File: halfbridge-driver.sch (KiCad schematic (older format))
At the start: 33 parts, among them U12 MGJ1, U13 MGJ1, U14 2ED020I12-F2

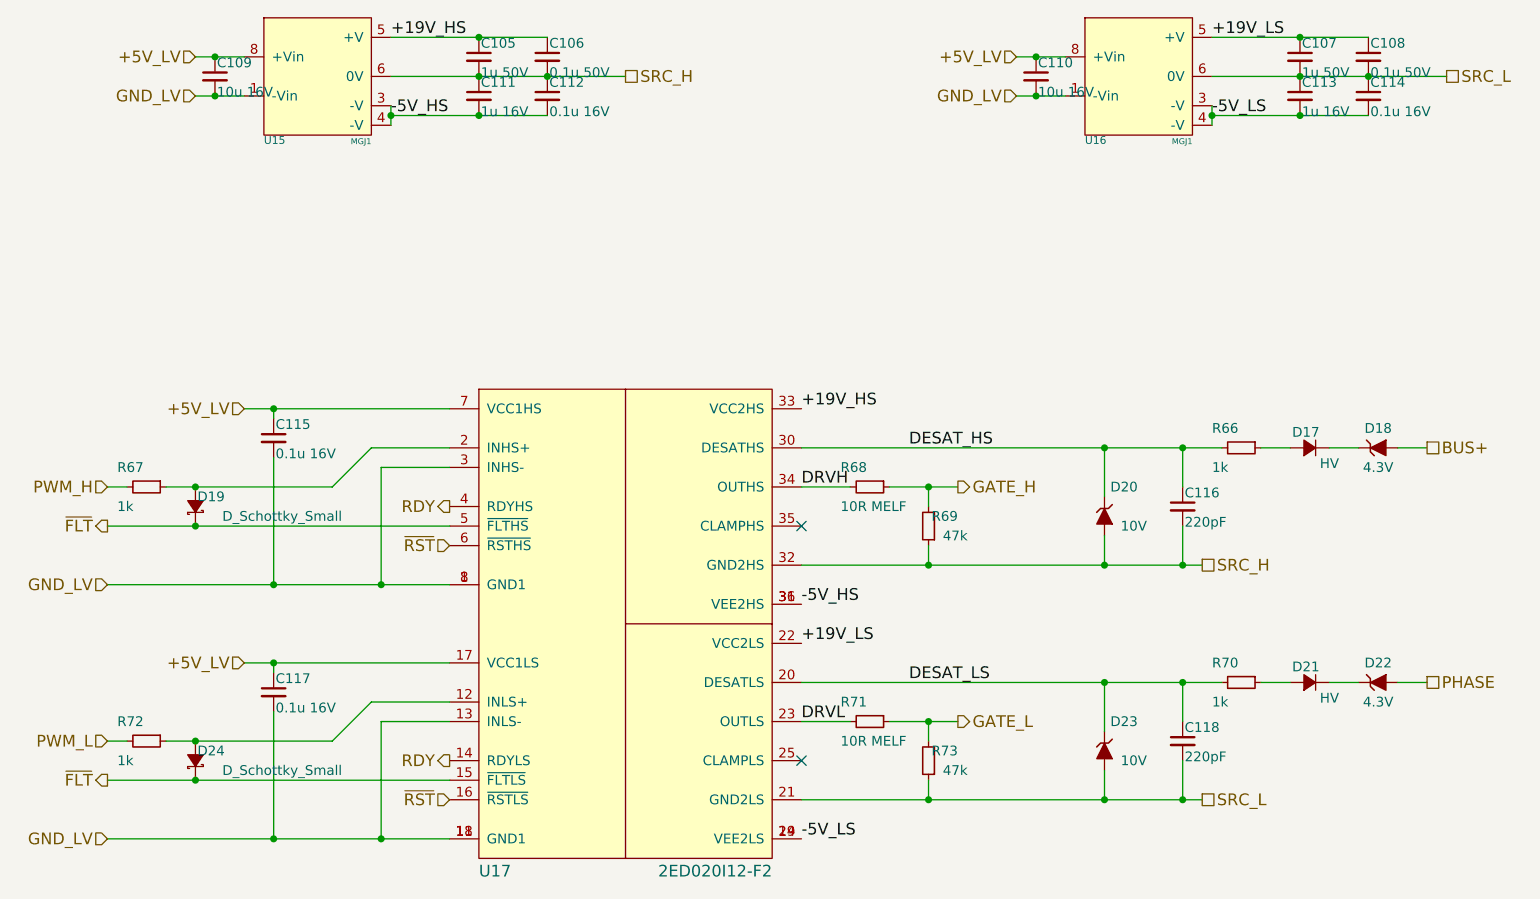
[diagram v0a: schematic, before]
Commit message: Add aux connector for vibe monitor
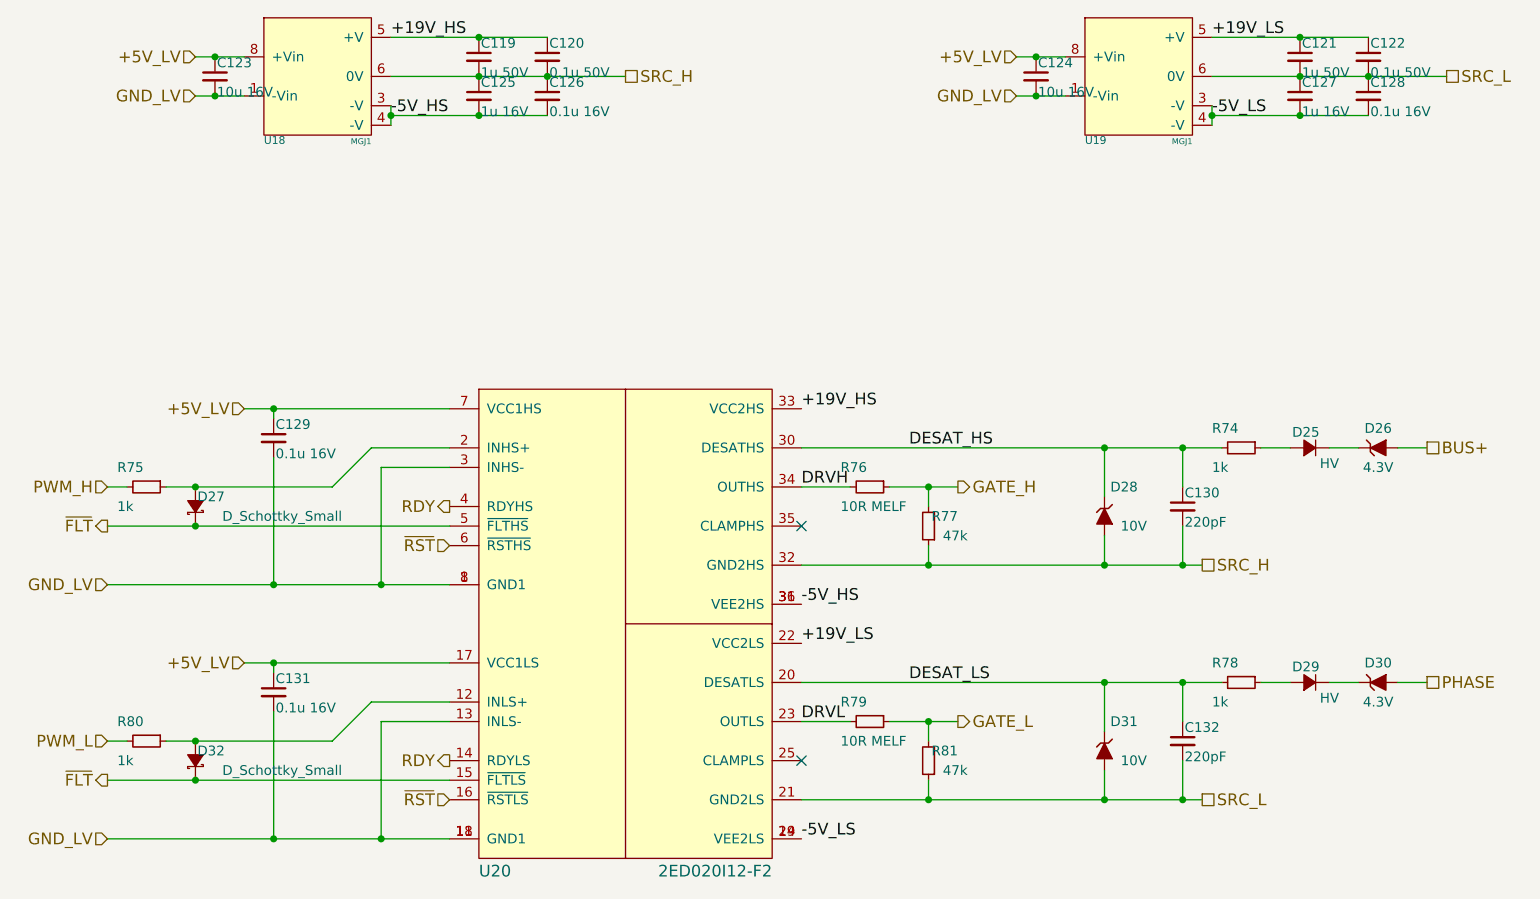
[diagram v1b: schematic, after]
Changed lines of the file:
@@
 AR Path="/57A1662D/57F260F4/57F02200" Ref="U17"  Part="1"
 AR Path="/57A1662D/57F2705F/57F02200" Ref="U20"  Part="1"
-F 0 "U17" H 4450 2750 60  0000 L BNN
+F 0 "U20" H 4450 2750 60  0000 L BNN
 F 1 "2ED020I12-F2" H 5950 2750 60  0000 R BNN
 F 2 "sictroller:PG-DSO-36-58" H 5200 4050 60  0001 C CNN
@@
 AR Path="/57A1662D/57F260F4/57F05C45" Ref="U15"  Part="1"
 AR Path="/57A1662D/57F2705F/57F05C45" Ref="U18"  Part="1"
-F 0 "U15" H 3350 900 40  0000 L BNN
+F 0 "U18" H 3350 900 40  0000 L BNN
 F 1 "MGJ1" H 3900 900 30  0000 R BNN
 F 2 "sictroller:MGJ1" H 3550 1250 60  0001 C CNN
@@
 AR Path="/57A1662D/57F260F4/57F05D03" Ref="C109"  Part="1"
 AR Path="/57A1662D/57F2705F/57F05D03" Ref="C123"  Part="1"
-F 0 "C109" H 3110 1320 50  0000 L CNN
+F 0 "C123" H 3110 1320 50  0000 L CNN
 F 1 "10u 16V" H 3110 1170 50  0000 L CNN
 F 2 "Capacitors_SMD:C_0805" H 3100 1250 50  0001 C CNN
@@
 AR Path="/57A1662D/57F260F4/57F05DBD" Ref="C105"  Part="1"
 AR Path="/57A1662D/57F2705F/57F05DBD" Ref="C119"  Part="1"
-F 0 "C105" H 4460 1220 50  0000 L CNN
+F 0 "C119" H 4460 1220 50  0000 L CNN
 F 1 "1u 50V" H 4460 1070 50  0000 L CNN
 F 2 "Capacitors_SMD:C_0805" H 4450 1150 50  0001 C CNN
@@
 AR Path="/57A1662D/57F260F4/57F05E19" Ref="C111"  Part="1"
 AR Path="/57A1662D/57F2705F/57F05E19" Ref="C125"  Part="1"
-F 0 "C111" H 4460 1420 50  0000 L CNN
+F 0 "C125" H 4460 1420 50  0000 L CNN
 F 1 "1u 16V" H 4460 1270 50  0000 L CNN
 F 2 "Capacitors_SMD:C_0603" H 4450 1350 50  0001 C CNN
@@
 AR Path="/57A1662D/57F260F4/57F0708D" Ref="U16"  Part="1"
 AR Path="/57A1662D/57F2705F/57F0708D" Ref="U19"  Part="1"
-F 0 "U16" H 7550 900 40  0000 L BNN
+F 0 "U19" H 7550 900 40  0000 L BNN
 F 1 "MGJ1" H 8100 900 30  0000 R BNN
 F 2 "sictroller:MGJ1" H 7750 1250 60  0001 C CNN
@@
 AR Path="/57A1662D/57F260F4/57F07093" Ref="C110"  Part="1"
 AR Path="/57A1662D/57F2705F/57F07093" Ref="C124"  Part="1"
-F 0 "C110" H 7310 1320 50  0000 L CNN
+F 0 "C124" H 7310 1320 50  0000 L CNN
 F 1 "10u 16V" H 7310 1170 50  0000 L CNN
 F 2 "Capacitors_SMD:C_0805" H 7300 1250 50  0001 C CNN
@@
 AR Path="/57A1662D/57F260F4/57F07099" Ref="C107"  Part="1"
 AR Path="/57A1662D/57F2705F/57F07099" Ref="C121"  Part="1"
-F 0 "C107" H 8660 1220 50  0000 L CNN
+F 0 "C121" H 8660 1220 50  0000 L CNN
 F 1 "1u 50V" H 8660 1070 50  0000 L CNN
 F 2 "Capacitors_SMD:C_0805" H 8650 1150 50  0001 C CNN
@@
 AR Path="/57A1662D/57F260F4/57F0709F" Ref="C113"  Part="1"
 AR Path="/57A1662D/57F2705F/57F0709F" Ref="C127"  Part="1"
-F 0 "C113" H 8660 1420 50  0000 L CNN
+F 0 "C127" H 8660 1420 50  0000 L CNN
 F 1 "1u 16V" H 8660 1270 50  0000 L CNN
 F 2 "Capacitors_SMD:C_0603" H 8650 1350 50  0001 C CNN
@@
 AR Path="/57A1662D/57F260F4/57F1574E" Ref="R68"  Part="1"
 AR Path="/57A1662D/57F2705F/57F1574E" Ref="R76"  Part="1"
-F 0 "R68" V 6350 3200 50  0000 L CNN
+F 0 "R76" V 6350 3200 50  0000 L CNN
 F 1 "10R MELF" V 6550 3200 50  0000 L CNN
 F 2 "sictroller:MELF-0204" H 6450 3350 50  0001 C CNN
@@
 AR Path="/57A1662D/57F260F4/57F16BC4" Ref="D17"  Part="1"
 AR Path="/57A1662D/57F2705F/57F16BC4" Ref="D25"  Part="1"
-F 0 "D17" H 8650 3230 50  0000 L CNN
+F 0 "D25" H 8650 3230 50  0000 L CNN
 F 1 "HV" H 8550 3070 50  0000 L CNN
 F 2 "Diodes_SMD:SMA_Standard" V 8700 3150 50  0001 C CNN
@@
 AR Path="/57A1662D/57F260F4/57F16C61" Ref="D18"  Part="1"
 AR Path="/57A1662D/57F2705F/57F16C61" Ref="D26"  Part="1"
-F 0 "D18" H 9050 3250 50  0000 C CNN
+F 0 "D26" H 9050 3250 50  0000 C CNN
 F 1 "4.3V" H 9050 3050 50  0000 C CNN
 F 2 "Diodes_SMD:SOD-523" H 9050 3150 50  0001 C CNN
@@
 AR Path="/57A1662D/57F260F4/57F16FB9" Ref="R66"  Part="1"
 AR Path="/57A1662D/57F2705F/57F16FB9" Ref="R74"  Part="1"
-F 0 "R66" V 8250 3000 50  0000 L CNN
+F 0 "R74" V 8250 3000 50  0000 L CNN
 F 1 "1k" V 8450 3000 50  0000 L CNN
 F 2 "Resistors_SMD:R_0402" H 8350 3150 50  0001 C CNN
@@
 AR Path="/57A1662D/57F260F4/57F17070" Ref="C116"  Part="1"
 AR Path="/57A1662D/57F2705F/57F17070" Ref="C130"  Part="1"
-F 0 "C116" H 8060 3520 50  0000 L CNN
+F 0 "C130" H 8060 3520 50  0000 L CNN
 F 1 "220pF" H 8060 3370 50  0000 L CNN
 F 2 "Capacitors_SMD:C_0402" H 8050 3450 50  0001 C CNN
@@
 AR Path="/57A1662D/57F260F4/57F185FE" Ref="R69"  Part="1"
 AR Path="/57A1662D/57F2705F/57F185FE" Ref="R77"  Part="1"
-F 0 "R69" H 6600 3500 50  0000 L CNN
+F 0 "R77" H 6600 3500 50  0000 L CNN
 F 1 "47k" H 6550 3600 50  0000 L CNN
 F 2 "Resistors_SMD:R_0805" H 6750 3550 50  0001 C CNN
@@
 AR Path="/57A1662D/57F260F4/57F1899B" Ref="D20"  Part="1"
 AR Path="/57A1662D/57F2705F/57F1899B" Ref="D28"  Part="1"
-F 0 "D20" V 7500 3600 50  0000 C CNN
+F 0 "D28" V 7500 3600 50  0000 C CNN
 F 1 "10V" V 7700 3650 50  0000 C CNN
 F 2 "Diodes_SMD:SOD-523" H 7650 3500 50  0001 C CNN
@@
 AR Path="/57A1662D/57F260F4/57F19BF8" Ref="R71"  Part="1"
 AR Path="/57A1662D/57F2705F/57F19BF8" Ref="R79"  Part="1"
-F 0 "R71" V 6350 4400 50  0000 L CNN
+F 0 "R79" V 6350 4400 50  0000 L CNN
 F 1 "10R MELF" V 6550 4400 50  0000 L CNN
 F 2 "sictroller:MELF-0204" H 6450 4550 50  0001 C CNN
@@
 AR Path="/57A1662D/57F260F4/57F19C08" Ref="D21"  Part="1"
 AR Path="/57A1662D/57F2705F/57F19C08" Ref="D29"  Part="1"
-F 0 "D21" H 8650 4430 50  0000 L CNN
+F 0 "D29" H 8650 4430 50  0000 L CNN
 F 1 "HV" H 8550 4270 50  0000 L CNN
 F 2 "Diodes_SMD:SMA_Standard" V 8700 4350 50  0001 C CNN
@@
 AR Path="/57A1662D/57F260F4/57F19C0E" Ref="D22"  Part="1"
 AR Path="/57A1662D/57F2705F/57F19C0E" Ref="D30"  Part="1"
-F 0 "D22" H 9050 4450 50  0000 C CNN
+F 0 "D30" H 9050 4450 50  0000 C CNN
 F 1 "4.3V" H 9050 4250 50  0000 C CNN
 F 2 "Diodes_SMD:SOD-523" H 9050 4350 50  0001 C CNN
@@
 AR Path="/57A1662D/57F260F4/57F19C16" Ref="R70"  Part="1"
 AR Path="/57A1662D/57F2705F/57F19C16" Ref="R78"  Part="1"
-F 0 "R70" V 8250 4200 50  0000 L CNN
+F 0 "R78" V 8250 4200 50  0000 L CNN
 F 1 "1k" V 8450 4200 50  0000 L CNN
 F 2 "Resistors_SMD:R_0402" H 8350 4350 50  0001 C CNN
@@
 AR Path="/57A1662D/57F260F4/57F19C1F" Ref="C118"  Part="1"
 AR Path="/57A1662D/57F2705F/57F19C1F" Ref="C132"  Part="1"
-F 0 "C118" H 8060 4720 50  0000 L CNN
+F 0 "C132" H 8060 4720 50  0000 L CNN
 F 1 "220pF" H 8060 4570 50  0000 L CNN
 F 2 "Capacitors_SMD:C_0402" H 8050 4650 50  0001 C CNN
@@
 AR Path="/57A1662D/57F260F4/57F19C2A" Ref="R73"  Part="1"
 AR Path="/57A1662D/57F2705F/57F19C2A" Ref="R81"  Part="1"
-F 0 "R73" H 6600 4700 50  0000 L CNN
+F 0 "R81" H 6600 4700 50  0000 L CNN
 F 1 "47k" H 6550 4800 50  0000 L CNN
 F 2 "Resistors_SMD:R_0805" H 6750 4750 50  0001 C CNN
@@
 AR Path="/57A1662D/57F260F4/57F19C34" Ref="D23"  Part="1"
 AR Path="/57A1662D/57F2705F/57F19C34" Ref="D31"  Part="1"
-F 0 "D23" V 7500 4800 50  0000 C CNN
+F 0 "D31" V 7500 4800 50  0000 C CNN
 F 1 "10V" V 7700 4850 50  0000 C CNN
 F 2 "Diodes_SMD:SOD-523" H 7650 4700 50  0001 C CNN
@@
 AR Path="/57A1662D/57F260F4/57F1A51C" Ref="C115"  Part="1"
 AR Path="/57A1662D/57F2705F/57F1A51C" Ref="C129"  Part="1"
-F 0 "C115" H 3410 3170 50  0000 L CNN
+F 0 "C129" H 3410 3170 50  0000 L CNN
 F 1 "0.1u 16V" H 3410 3020 50  0000 L CNN
 F 2 "Capacitors_SMD:C_0402" H 3400 3100 50  0001 C CNN
@@
 AR Path="/57A1662D/57F260F4/57F1C1CA" Ref="R67"  Part="1"
 AR Path="/57A1662D/57F2705F/57F1C1CA" Ref="R75"  Part="1"
-F 0 "R67" V 2650 3200 50  0000 L CNN
+F 0 "R75" V 2650 3200 50  0000 L CNN
 F 1 "1k" V 2850 3200 50  0000 L CNN
 F 2 "Resistors_SMD:R_0402" H 2750 3350 50  0001 C CNN
@@
 AR Path="/57A1662D/57F260F4/57F1C51E" Ref="D19"  Part="1"
 AR Path="/57A1662D/57F2705F/57F1C51E" Ref="D27"  Part="1"
-F 0 "D19" V 3050 3300 50  0000 L CNN
+F 0 "D27" V 3050 3300 50  0000 L CNN
 F 1 "D_Schottky_Small" V 2950 2700 50  0000 L CNN
 F 2 "Diodes_SMD:SOD-523" V 3000 3450 50  0001 C CNN
@@
 AR Path="/57A1662D/57F260F4/57F1DED1" Ref="C117"  Part="1"
 AR Path="/57A1662D/57F2705F/57F1DED1" Ref="C131"  Part="1"
-F 0 "C117" H 3410 4470 50  0000 L CNN
+F 0 "C131" H 3410 4470 50  0000 L CNN
 F 1 "0.1u 16V" H 3410 4320 50  0000 L CNN
 F 2 "Capacitors_SMD:C_0402" H 3400 4400 50  0001 C CNN
@@
 AR Path="/57A1662D/57F260F4/57F1DEE0" Ref="R72"  Part="1"
 AR Path="/57A1662D/57F2705F/57F1DEE0" Ref="R80"  Part="1"
-F 0 "R72" V 2650 4500 50  0000 L CNN
+F 0 "R80" V 2650 4500 50  0000 L CNN
 F 1 "1k" V 2850 4500 50  0000 L CNN
 F 2 "Resistors_SMD:R_0402" H 2750 4650 50  0001 C CNN
@@
 AR Path="/57A1662D/57F260F4/57F1DEE7" Ref="D24"  Part="1"
 AR Path="/57A1662D/57F2705F/57F1DEE7" Ref="D32"  Part="1"
-F 0 "D24" V 3050 4600 50  0000 L CNN
+F 0 "D32" V 3050 4600 50  0000 L CNN
 F 1 "D_Schottky_Small" V 2950 4000 50  0000 L CNN
 F 2 "Diodes_SMD:SOD-523" V 3000 4750 50  0001 C CNN
@@
 AR Path="/57A1662D/57F260F4/57FC6B04" Ref="C108"  Part="1"
 AR Path="/57A1662D/57F2705F/57FC6B04" Ref="C122"  Part="1"
-F 0 "C108" H 9010 1220 50  0000 L CNN
+F 0 "C122" H 9010 1220 50  0000 L CNN
 F 1 "0.1u 50V" H 9010 1070 50  0000 L CNN
 F 2 "Capacitors_SMD:C_0603" H 9000 1150 50  0001 C CNN
@@
 AR Path="/57A1662D/57F260F4/57FC6BF3" Ref="C114"  Part="1"
 AR Path="/57A1662D/57F2705F/57FC6BF3" Ref="C128"  Part="1"
-F 0 "C114" H 9010 1420 50  0000 L CNN
+F 0 "C128" H 9010 1420 50  0000 L CNN
 F 1 "0.1u 16V" H 9010 1270 50  0000 L CNN
 F 2 "Capacitors_SMD:C_0402" H 9000 1350 50  0001 C CNN
@@
 AR Path="/57A1662D/57F260F4/57FC72B1" Ref="C106"  Part="1"
 AR Path="/57A1662D/57F2705F/57FC72B1" Ref="C120"  Part="1"
-F 0 "C106" H 4810 1220 50  0000 L CNN
+F 0 "C120" H 4810 1220 50  0000 L CNN
 F 1 "0.1u 50V" H 4810 1070 50  0000 L CNN
 F 2 "Capacitors_SMD:C_0603" H 4800 1150 50  0001 C CNN
@@
 AR Path="/57A1662D/57F260F4/57FC72B7" Ref="C112"  Part="1"
 AR Path="/57A1662D/57F2705F/57FC72B7" Ref="C126"  Part="1"
-F 0 "C112" H 4810 1420 50  0000 L CNN
+F 0 "C126" H 4810 1420 50  0000 L CNN
 F 1 "0.1u 16V" H 4810 1270 50  0000 L CNN
 F 2 "Capacitors_SMD:C_0402" H 4800 1350 50  0001 C CNN
